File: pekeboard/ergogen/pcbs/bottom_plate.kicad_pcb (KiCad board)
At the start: 2 copper layers, 150.9 x 124.7 mm, 0 parts

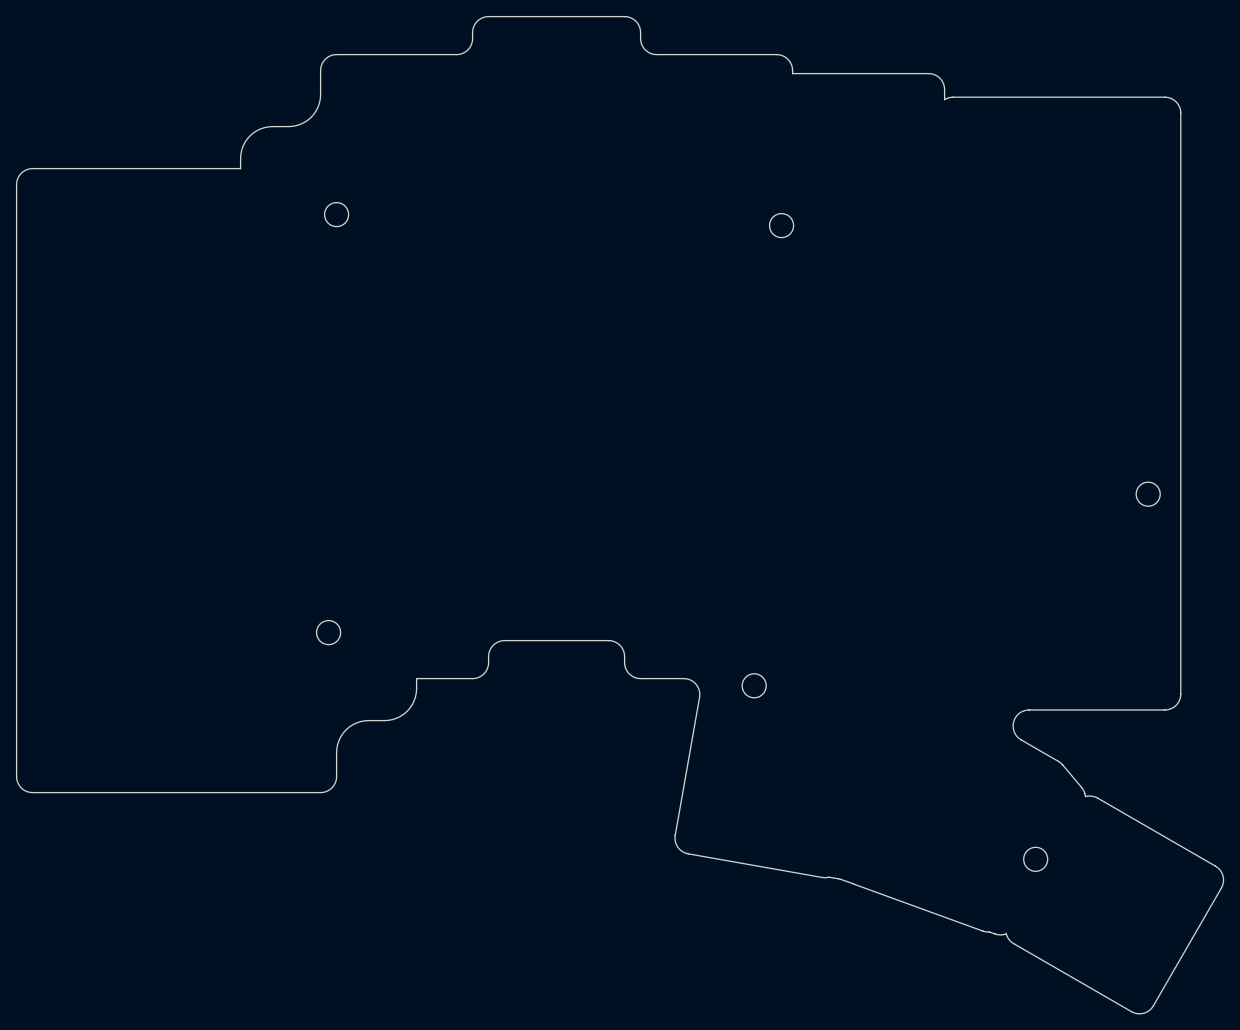
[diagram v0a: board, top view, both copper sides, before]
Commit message: pekepad folder fix
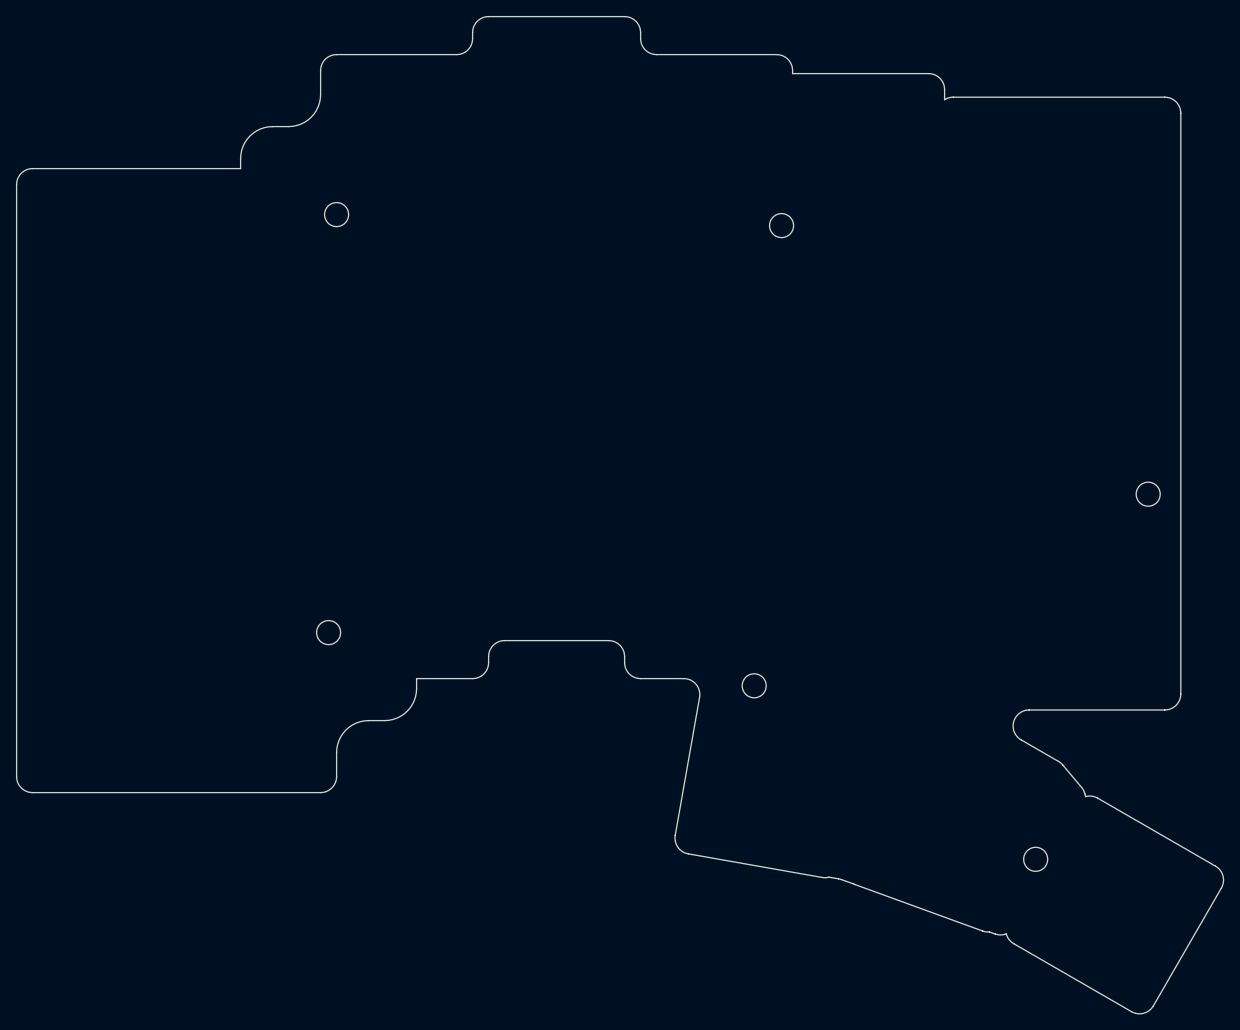
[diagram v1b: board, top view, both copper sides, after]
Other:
- outline, holes or cut-outs redrawn
